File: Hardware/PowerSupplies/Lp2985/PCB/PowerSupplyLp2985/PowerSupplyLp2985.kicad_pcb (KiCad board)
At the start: 2 copper layers, 7 parts, among them J1 Barrel_Jack, J2 Conn_01x02_Pin, U1 LP2985-5.0

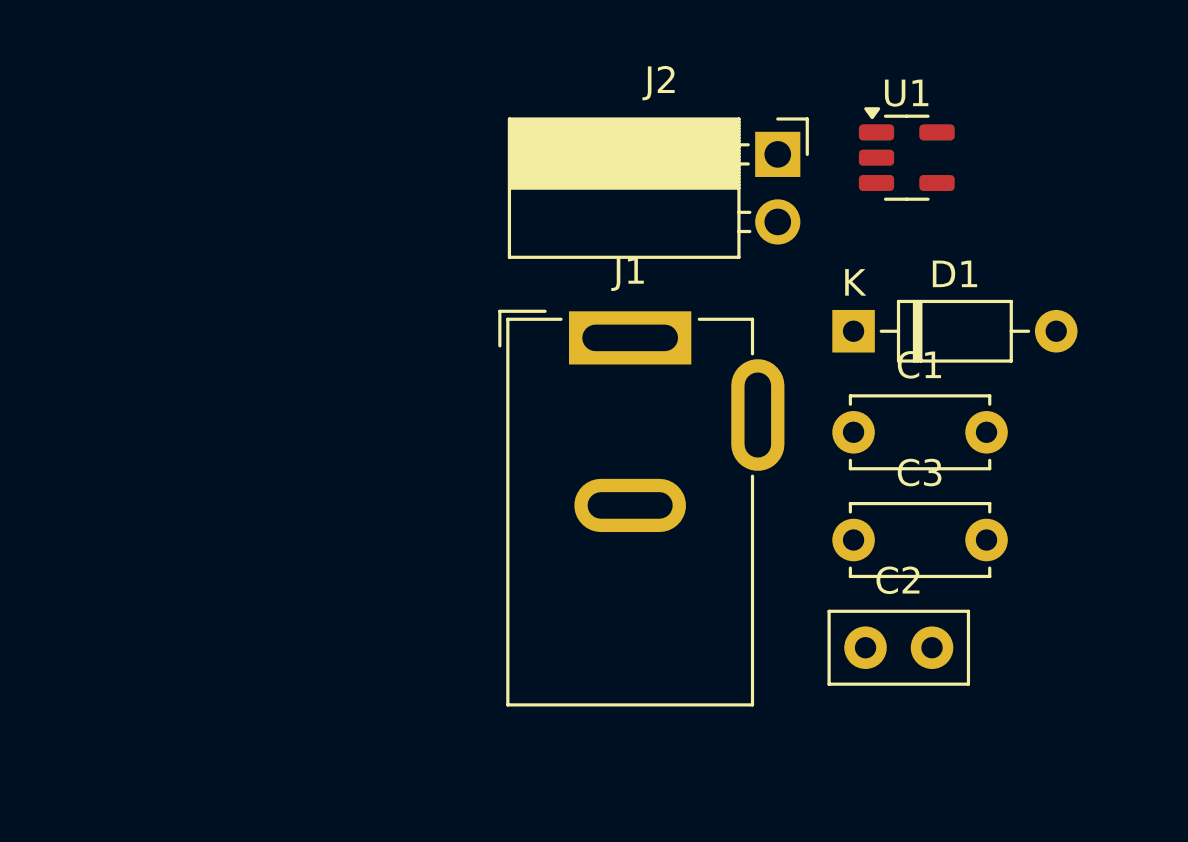
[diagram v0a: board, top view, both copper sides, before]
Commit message: Added consistency
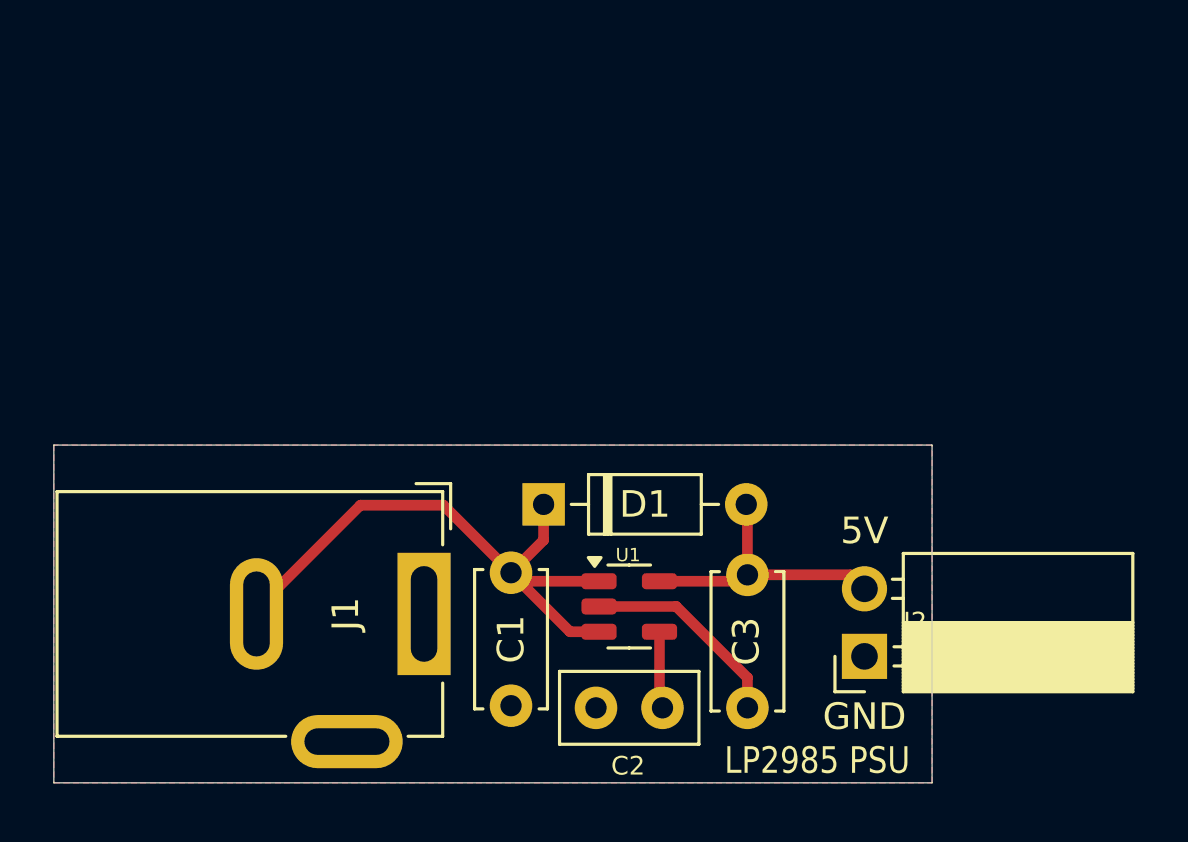
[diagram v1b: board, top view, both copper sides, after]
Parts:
- moved U1 19.8 mm to (97.8, 81.0)
- moved J2 19.2 mm to (106.7, 82.9), turned to 180 degrees
- moved C1 13.9 mm to (93.4, 79.7), turned to -90 degrees
- moved D1 13.3 mm to (94.6, 77.2)
- moved J1 13.0 mm to (90.1, 81.3), turned to -90 degrees
- moved C2 10.4 mm to (96.6, 84.8)
- moved C3 4.20 mm to (102.3, 79.8), turned to -90 degrees
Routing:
- net /2.5-16V: track 0.00 -> 22.6 mm
- net /5V: track 0.00 -> 10.9 mm
- net GND: track 0.00 -> 7.82 mm
- net Net-(U1-BP): track 0.00 -> 2.91 mm
- added copper zone on F.Cu, net GND
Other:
- board outline added: 33 x 12.7 mm
- board text added: "5V"
- board text added: "GND"
- board text added: "LP2985 PSU"
